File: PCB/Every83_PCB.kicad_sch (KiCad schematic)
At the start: 36 parts, among them IC2 GD25Q16, J1 781710004, J2 Conn_01x08_Pin, J3 Conn_ARM_SWD_TagConnect_TC203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, Q3 DMG2305, SW101 KMR2, SW102 KMR2, U2 AP2112(3.3V), U3 MCP73831T-2ACI/OT, X3 JSTPH, Y2 32.768

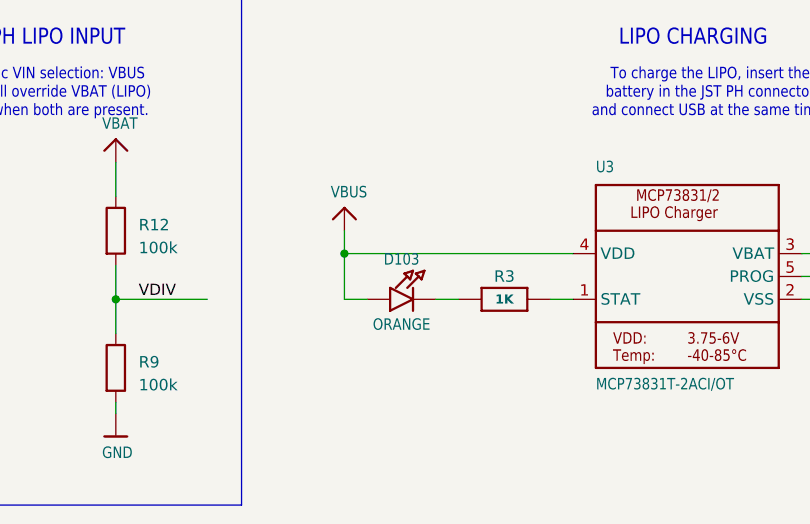
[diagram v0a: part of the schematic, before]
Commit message: WIP
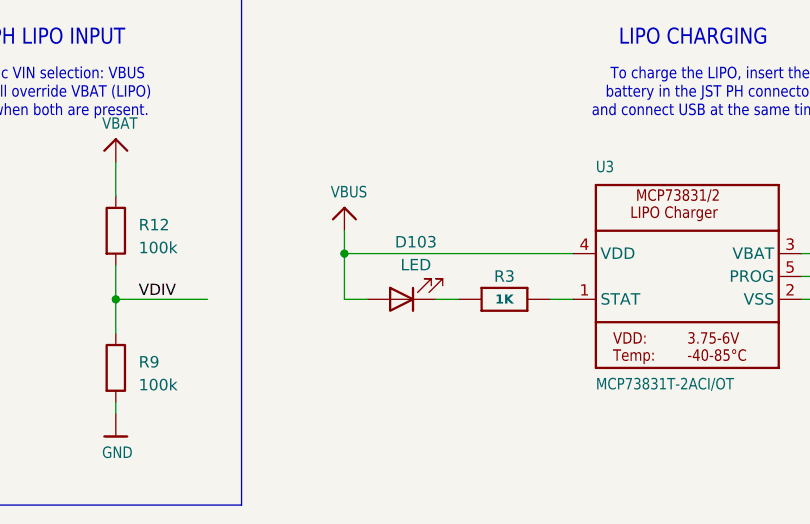
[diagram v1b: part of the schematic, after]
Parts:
- removed D103: ORANGE, Adafruit nRF52840 Bluefruit Feather Express Rev D:CHIPLED_0805_NOOUTLINE, symbol Adafruit nRF52840 Bluefruit Feather Express Rev D-eagle-import:LED0805_NOOUTLINE
- added D103: LED, Diode_SMD:D_0805_2012Metric_Pad1.15x1.40mm_HandSolder, symbol Device:LED
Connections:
- net VBUS: now also D103.2 (A)
- net at R3.1: now also D103.1 (K)
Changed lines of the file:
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@@
-    )
-  )
-  (symbol (lib_id "Adafruit nRF52840 Bluefruit Feather Express Rev D-eagle-import:LED0805_NOOUTLINE") (at 228.6 246.38 0) (unit 1)
-    (in_bom yes) (on_board yes) (dnp no)
-    (property "Reference" "D103" (at 227.33 241.935 0)
-      (effects (font (size 1.27 1.0795)))
-    )
-    (property "Value" "ORANGE" (at 227.33 249.174 0)
-      (effects (font (size 1.27 1.0795)))
-    )
-    (property "Footprint" "Adafruit nRF52840 Bluefruit Feather Express Rev D:CHIPLED_0805_NOOUTLINE" (at 228.6 246.38 0)
-      (effects (font (size 1.27 1.27)) hide)
-    )
-    (property "Datasheet" "" (at 228.6 246.38 0)
-      (effects (font (size 1.27 1.27)) hide)
-    )
-    (pin "A")
-    (pin "C")
-    (instances
-      (project "Every83_PCB"
-        (path "/ea2432c4-eb7a-431a-b465-8c00cfcb4450"
-          (reference "D103") (unit 1)
-        )
-      )
     )
   )
@@
         )
       )
+    )
+  )
+  (symbol (lib_id "Device:LED") (at 227.33 246.38 180) (unit 1)
+    (in_bom yes) (on_board yes) (dnp no) (fields_autoplaced)
+    (property "Reference" "D103" (at 228.9175 240.03 0)
+      (effects (font (size 1.27 1.27)))
+    )
+    (property "Value" "LED" (at 228.9175 242.57 0)
+      (effects (font (size 1.27 1.27)))
+    )
+    (property "Footprint" "Diode_SMD:D_0805_2012Metric_Pad1.15x1.40mm_HandSolder" (at 227.33 246.38 0)
+      (effects (font (size 1.27 1.27)) hide)
+    )
+    (property "Datasheet" "~" (at 227.33 246.38 0)
+      (effects (font (size 1.27 1.27)) hide)
+    )
+    (pin "1")
+    (pin "2")
+    (instances
+      (project "Every83_PCB"
+        (path "/ea2432c4-eb7a-431a-b465-8c00cfcb4450"
+          (reference "D103") (unit 1)
+        )
+      )
